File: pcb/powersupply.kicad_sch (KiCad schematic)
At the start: 21 parts, among them U4 AMS1117-3.3, U5 SMAJ18A-TR, U5 TPS54302

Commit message: stepdown L and layout further optimized. fix rotation and layout
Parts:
- L13: footprint Inductor_SMD:L_12x12mm_H4.5mm -> Inductor_SMD:L_6.3x6.3_H3; LCSC C5127462 -> C408412; LINK https://jlcpcb.com/partdetail/LantuMicro-SMS1050100MT/C5127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 -> https://jlcpcb.com/partdetail/Sunlord-MWSA0503S100MT/C408412
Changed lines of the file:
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@@
       (effects (font (size 1.27 1.27)))
     )
-    (property "Footprint" "Inductor_SMD:L_12x12mm_H4.5mm" (at 124.46 46.99 0)
+    (property "Footprint" "Inductor_SMD:L_6.3x6.3_H3" (at 124.46 46.99 0)
       (effects (font (size 1.27 1.27)) hide)
     )
@@
       (effects (font (size 1.27 1.27)) hide)
     )
-    (property "LCSC" "C5127462" (at 124.46 46.99 90)
+    (property "LCSC" "C408412" (at 124.46 46.99 90)
       (effects (font (size 1.27 1.27)) hide)
     )
-    (property "LINK" "https://jlcpcb.com/partdetail/LantuMicro-SMS1050100MT/C5127462" (at 124.46 46.99 0)
+    (property "LINK" "https://jlcpcb.com/partdetail/Sunlord-MWSA0503S100MT/C408412" (at 124.46 46.99 0)
       (effects (font (size 1.27 1.27)) hide)
     )

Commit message: fix: for the big elcap, use jlc part C3445244 to avoid running into expensive standard service
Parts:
- C57: LCSC C4747956 -> C3445244; LINK https://jlcpcb.com/partdetail/Knscha-RST470UF25V032/C4747956 -> https://jlcpcb.com/parts/componentSearch?searchTxt=C3445244
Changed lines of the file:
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@@
       (effects (font (size 1.27 1.27)) hide)
     )
-    (property "LCSC" "C4747956" (at 53.34 54.61 0)
+    (property "LCSC" "C3445244" (at 53.34 54.61 0)
       (effects (font (size 1.27 1.27)) hide)
     )
-    (property "LINK" "https://jlcpcb.com/partdetail/Knscha-RST470UF25V032/C4747956" (at 53.34 54.61 0)
+    (property "LINK" "https://jlcpcb.com/parts/componentSearch?searchTxt=C3445244" (at 53.34 54.61 0)
       (effects (font (size 1.27 1.27)) hide)
     )

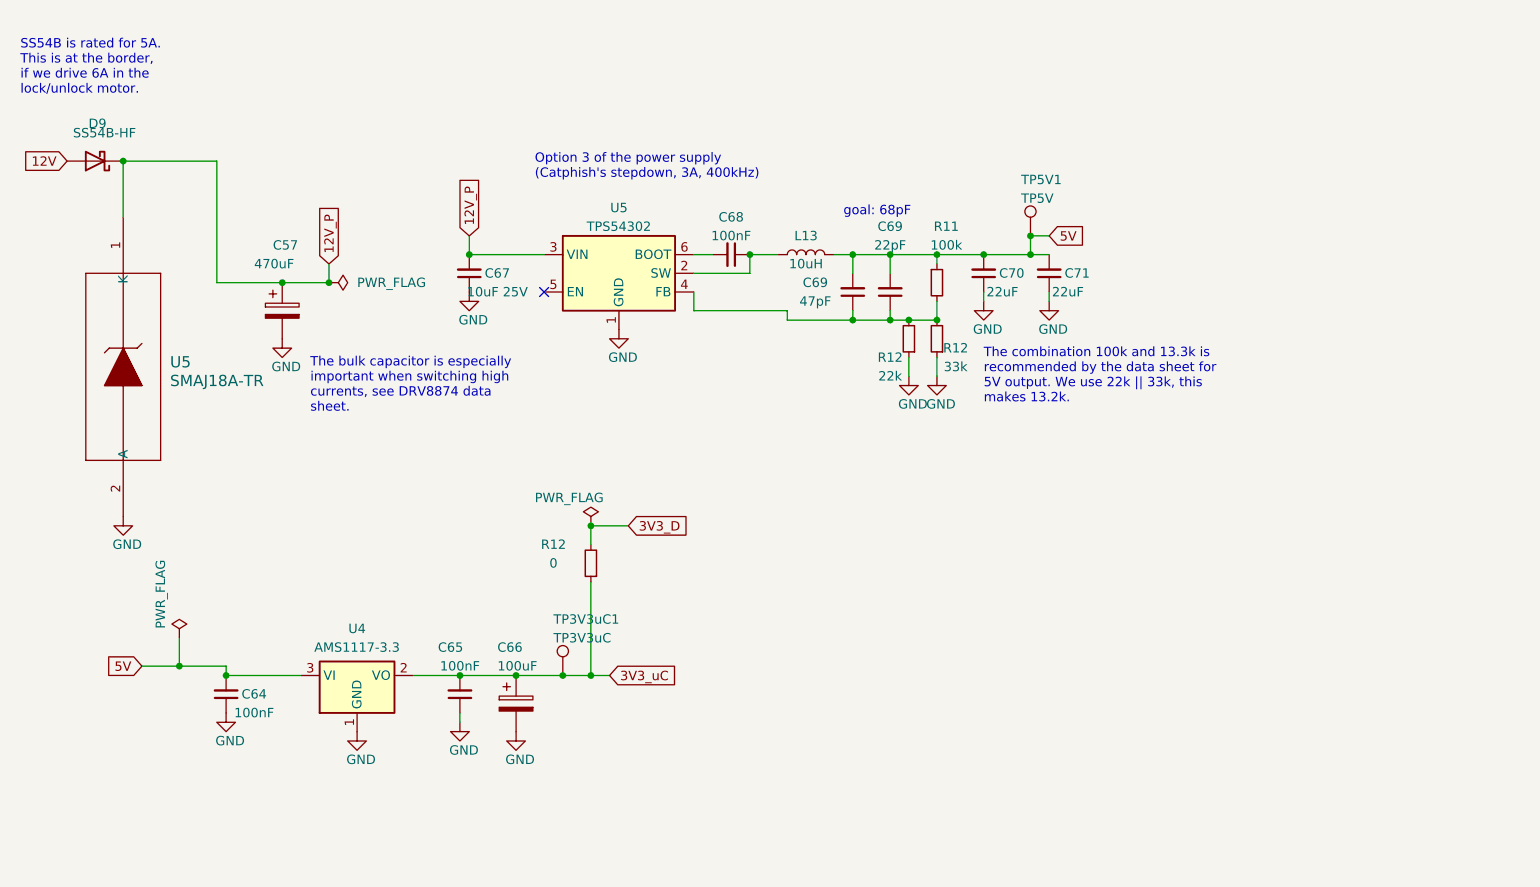
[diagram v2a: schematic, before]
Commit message: feature: Added wakeup logic
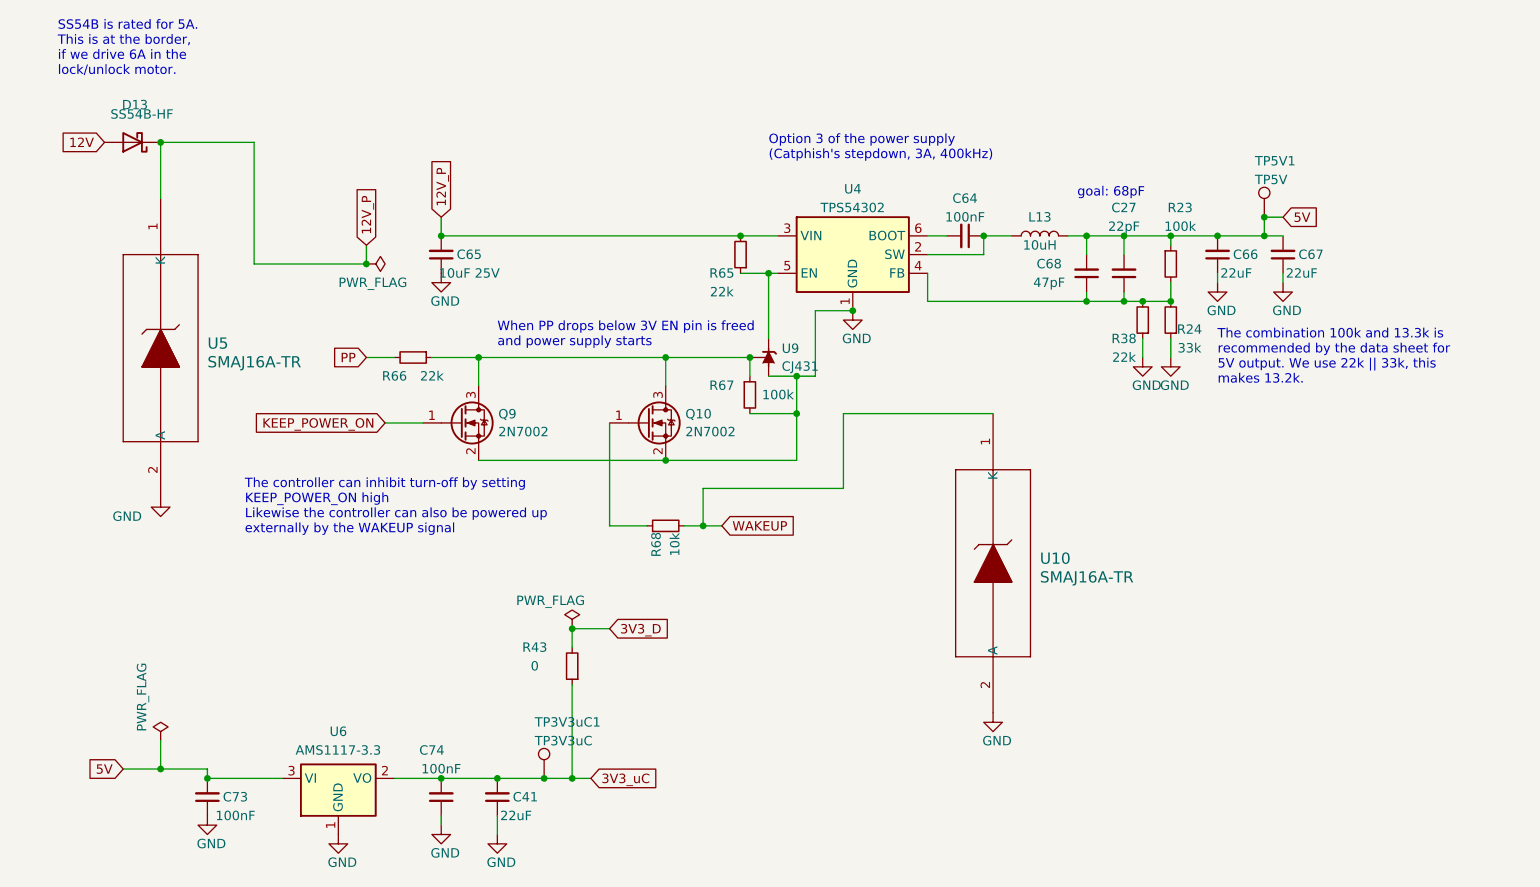
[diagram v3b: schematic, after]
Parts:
- removed C57: 470uF, Capacitor_SMD:CP_Elec_10x10, symbol Device:C_Polarized
- removed C66: 100uF, Capacitor_SMD:CP_Elec_8x10, symbol Device:C_Polarized
- added C41: 22uF, Capacitor_SMD:C_1210_3225Metric_Pad1.33x2.70mm_HandSolder, symbol Device:C_Small
- added Q10, Q9: 2N7002, Package_TO_SOT_SMD:SOT-23, symbol Transistor_FET:2N7002
- added R65, R66: 22k, Resistor_SMD:R_0805_2012Metric_Pad1.20x1.40mm_HandSolder, symbol Device:R_Small
- added R67: 100k, Resistor_SMD:R_0805_2012Metric_Pad1.20x1.40mm_HandSolder, symbol Device:R_Small
- added R68: 10k, Resistor_SMD:R_0805_2012Metric_Pad1.20x1.40mm_HandSolder, symbol Device:R_Small
- added U10: SMAJ16A-TR, tvs:SMA_UNI_STM, symbol TVS:SMAJ18A-TR
- added U9: CJ431, Package_TO_SOT_SMD:SOT-23-3, symbol Reference_Voltage:TL431DBZ
- U5: value SMAJ18A-TR -> SMAJ16A-TR; footprint SMA_UNI_STM -> tvs:SMA_UNI_STM; LCSC C908771 -> C908770
- renumbered C69 to C27, C68 to C64, C67 to C65, C70 to C66, C71 to C67, C69 to C68, C64 to C73, C65 to C74, D9 to D13, R11 to R23, R12 to R24, R12 to R38, R12 to R43, U5 to U4, U4 to U6
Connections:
- net 12V_P: now also R65.2
- net 3V3_uC: now also C41.2
- net GND: now also C41.1, Q10.2 (S), Q9.2 (S), R67.2, U10.2 (A), U9.3 (A)
- net at U4.5 (EN): now also R65.1, U9.1 (K)
- new net: Q10.3 (D), Q9.3 (D), R66.1, R67.1, U9.2 (REF)
- new net: Q10.1 (G), R68.1
- new net KEEP_POWER_ON: Q9.1 (G)
- new net PP: R66.2
- new net WAKEUP: R68.2, U10.1 (K)
- no-connect marks 1 -> 0
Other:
- note added: "The controller can inhibit turn-off by setting KEEP_POWER_ON high Likewise the controller can also be powered up externally by the WAKEUP signal"
- note added: "When PP drops below 3V EN pin is freed and power supply starts"
- note removed: "The bulk capacitor is especially important when switching high currents, see DRV8874 data sheet."
- moved on the sheet: C27, C64, C65, C66, C67, C68, C73, C74, D13, L13, R23, R24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
